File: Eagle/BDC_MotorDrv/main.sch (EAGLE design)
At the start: 8 parts, among them U1 ATTINY10-TSHR

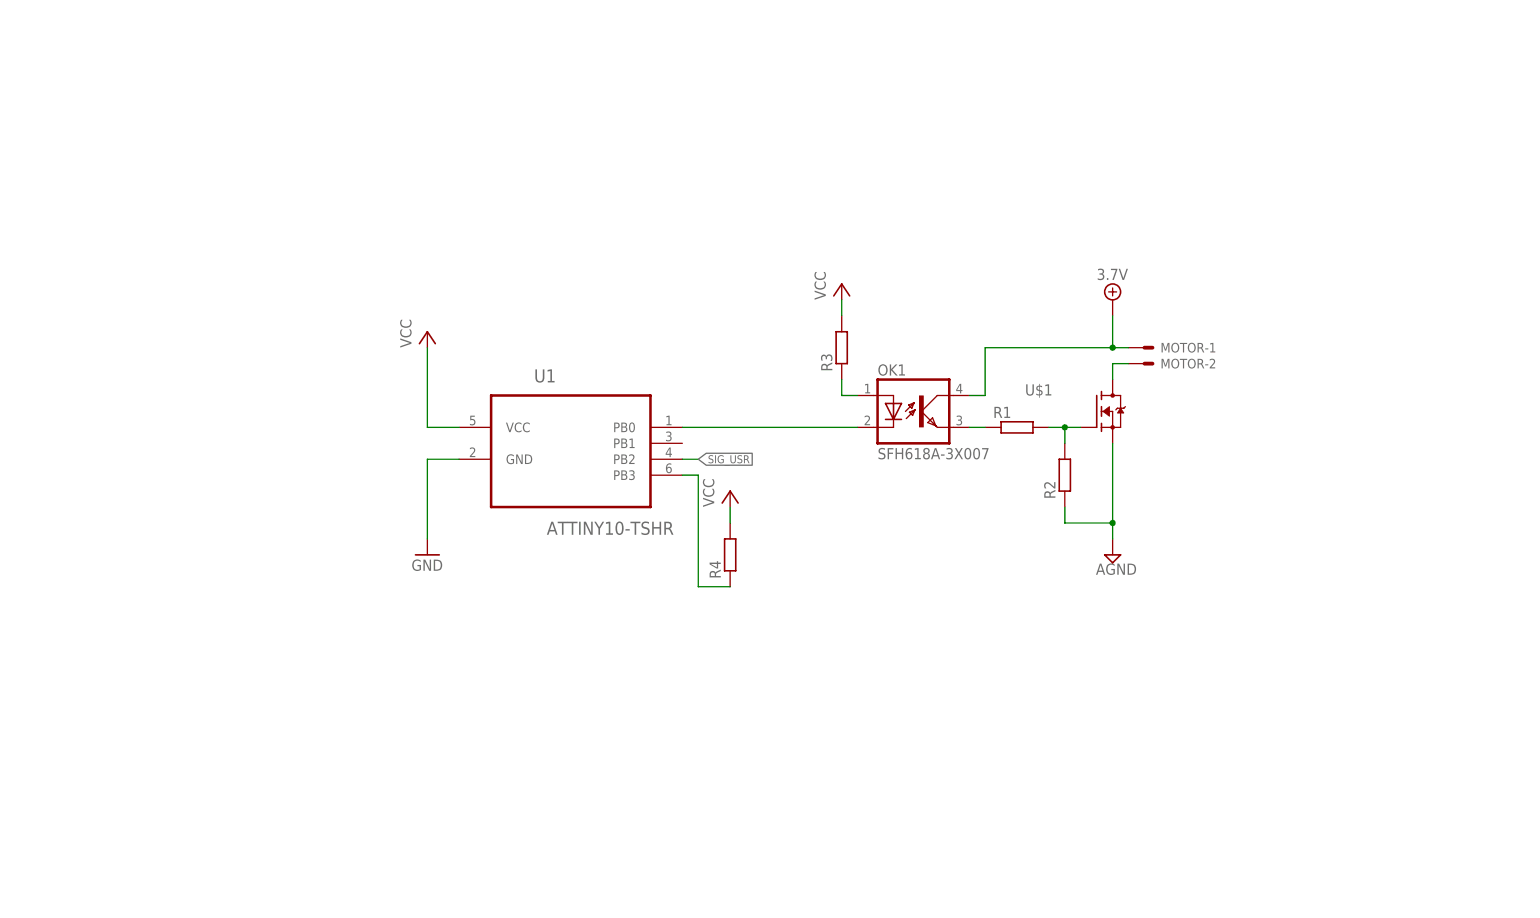
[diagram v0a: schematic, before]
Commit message: First version of schematic finished
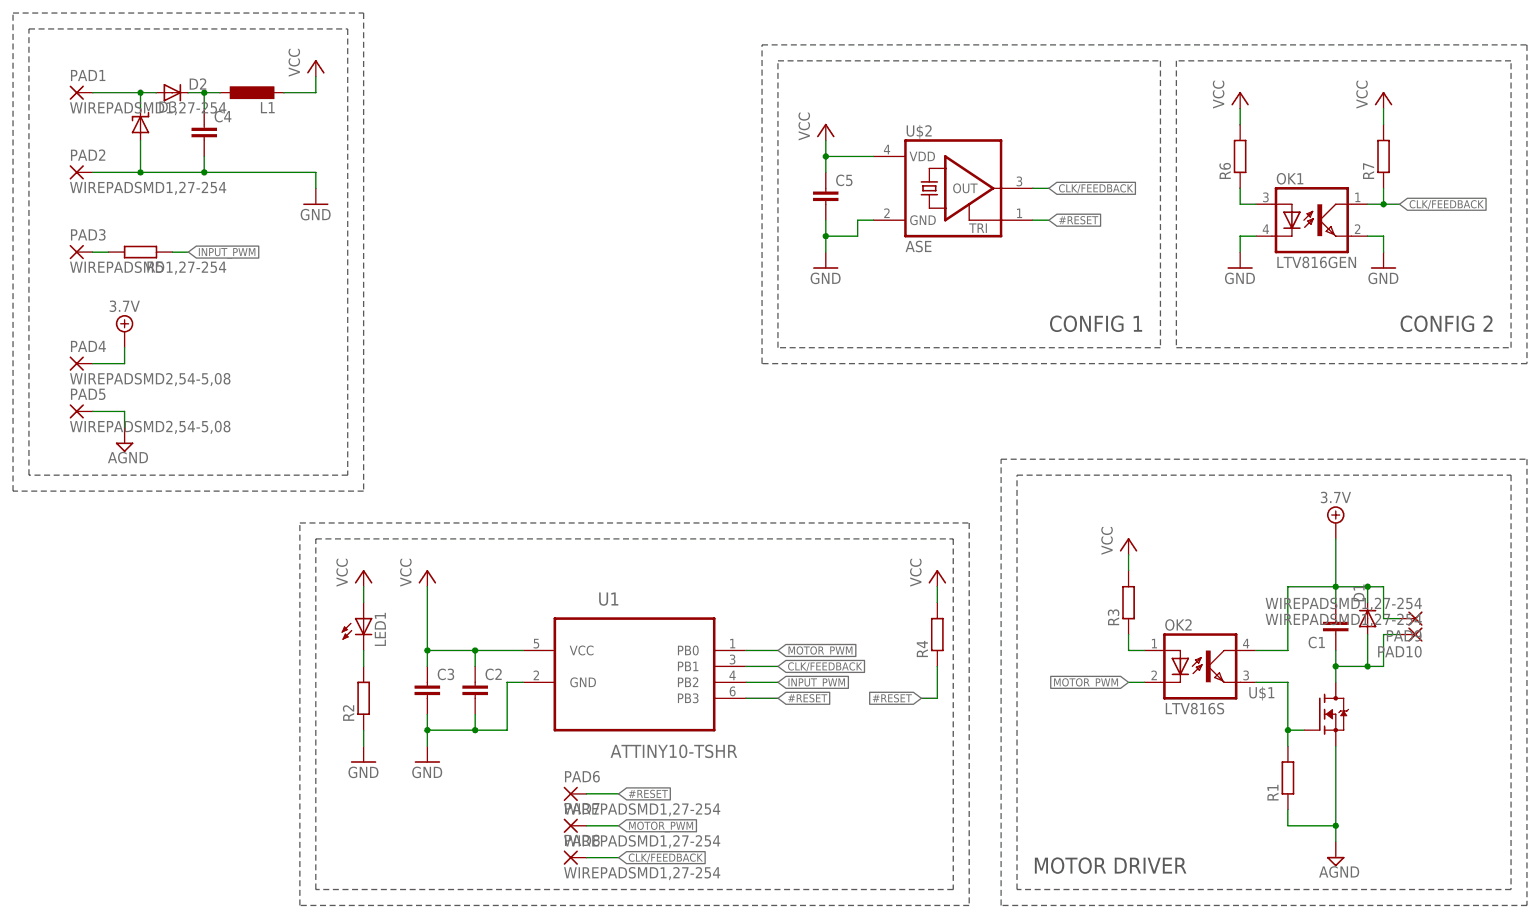
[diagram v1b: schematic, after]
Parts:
- removed MOTOR: 22-23-2021, con-molex:22-23-2021
- added C1, C3, C4, C5: (no value), rcl:C-EUC0603K
- added C2: (no value), rcl:C-EUC1206K
- added D1, D2: (no value), diode:DIODE-MINIMELF
- added D3: (no value), diode:SUPPRESSOR-SMBJ
- added L1: (no value), rcl:L-EUL2012C
- added LED1: (no value), led:LEDSML0603
- added OK2: LTV816S, optocoupler:LTV816S
- added PAD1, PAD10, PAD2, PAD3, PAD6, PAD7, PAD8, PAD9: WIREPADSMD1,27-254, wirepad:WIREPADSMD1,27-254
- added PAD4, PAD5: WIREPADSMD2,54-5,08, wirepad:WIREPADSMD2,54-5,08
- added R5, R6, R7: (no value), rcl:R-EU_R0603
- added U$2: ASE, crystal:ASE
- OK1: value SFH618A-3X007 -> LTV816GEN; device optocoupler:SFH618A-3X007 -> optocoupler:LTV816GEN
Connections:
- removed net N$6: R4.1, U1.PB3
- removed net SIG_USR: U1.PB2
- new net #RESET: PAD6.P, R4.1, U$2.TRI, U1.PB3
- new net CLK/FEEDBACK: OK1.COL, PAD8.P, R7.1, U$2.OUT, U1.PB1
- new net INPUT_PWM: R5.1, U1.PB2
- new net MOTOR_PWM: OK2.C, PAD7.P, U1.PB0
- new net N$10: LED1.C, R2.2
- new net N$13: PAD3.P, R5.2
- new net N$7: OK2.EMIT, R1.2, U$1.G
- net +12V: now also C1.2, D1.C, OK2.COL, PAD4.P, PAD9.P; no longer MOTOR-1.S, OK1.COL
- net AGND: now also PAD5.P, R1.1; no longer R2.1
- net GND: now also C2.2, C3.2, C4.2, C5.2, D3.A, OK1.C, OK1.EMIT, PAD2.P, R2.1, U$2.GND
- net N$1: now also OK2.A; no longer OK1.A
- net N$2: now also OK1.A, R6.1; no longer OK1.C, U1.PB0
- net N$3: now also D2.A, D3.C, PAD1.P; no longer R1.2, R2.2, U$1.G
- net N$4: now also C1.1, D1.A, PAD10.P; no longer MOTOR-2.S
- net N$5: now also C4.1, D2.C, L1.1; no longer OK1.EMIT, R1.1
- net VCC: now also C2.1, C3.1, C5.1, L1.2, LED1.A, R6.2, R7.2, U$2.VDD
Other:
- note added: "CONFIG 1"
- note added: "CONFIG 2"
- note added: "MOTOR DRIVER"
- moved on the sheet: OK1, R1, R2, R3, R4, U$1, U1
